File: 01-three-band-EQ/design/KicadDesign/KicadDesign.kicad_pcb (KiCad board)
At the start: 2 copper layers, 101 x 80.9 mm, 34 parts, among them J2 Output, J3 Input, J4 Supply, U1 TL072, U2 TL072, U3 TL072

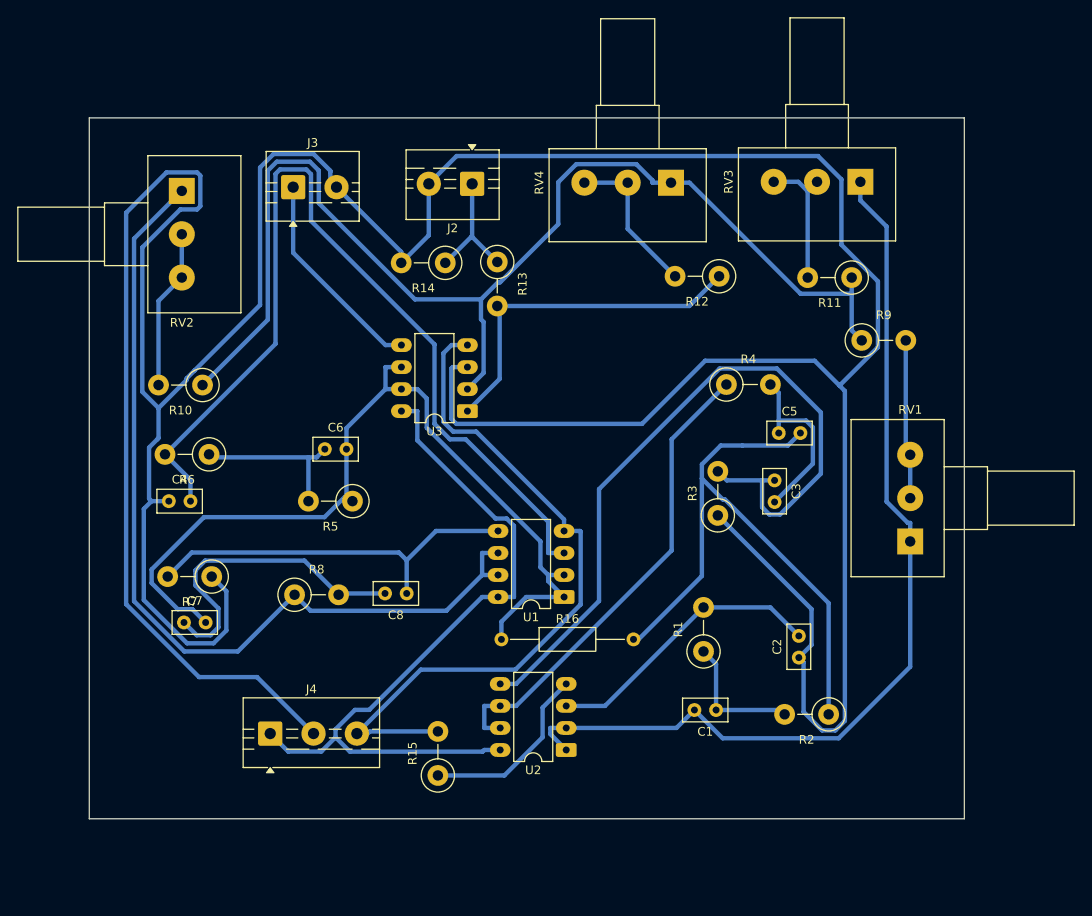
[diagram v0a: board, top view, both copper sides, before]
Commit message: feat: PCB routed
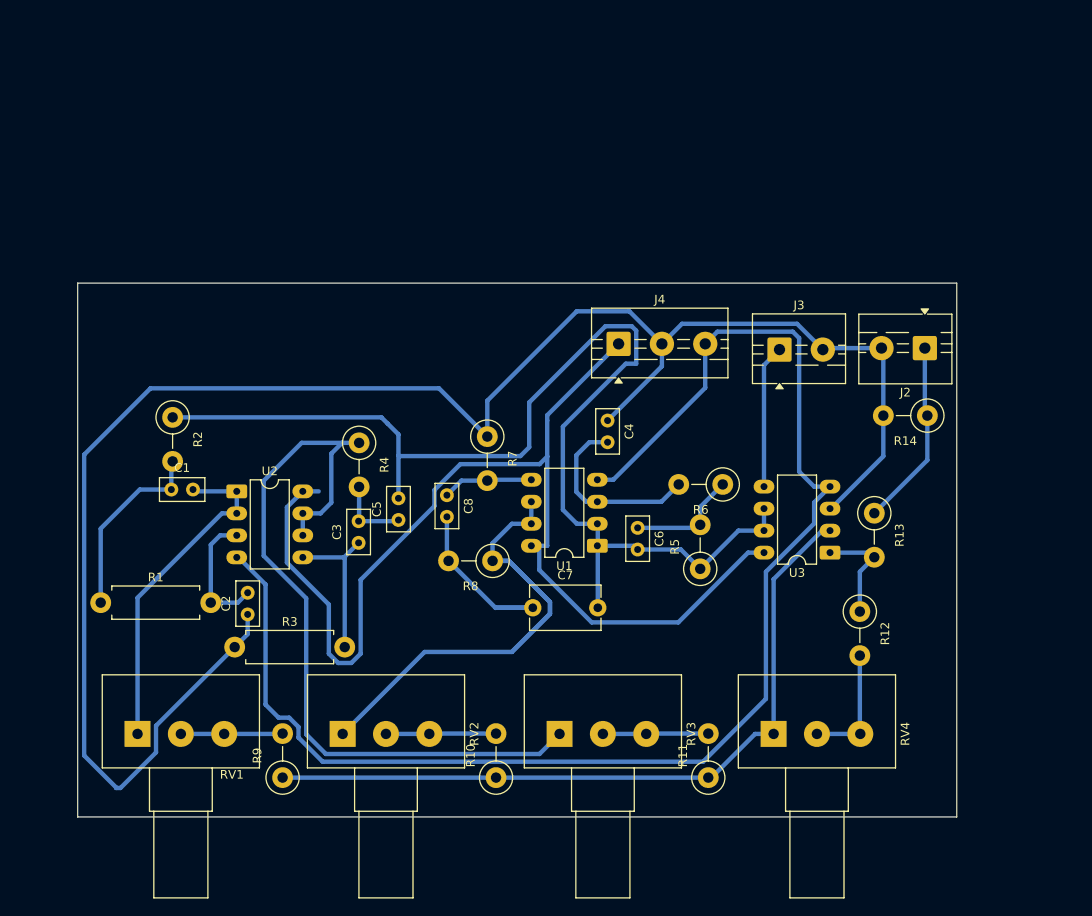
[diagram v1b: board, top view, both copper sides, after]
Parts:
- removed R15: 0, Resistor_THT:R_Axial_DIN0411_L9.9mm_D3.6mm_P5.08mm_Vertical
- removed R16: 270k, Resistor_THT:R_Axial_DIN0207_L6.3mm_D2.5mm_P15.24mm_Horizontal
- C7: footprint Capacitor_THT:C_Disc_D5.0mm_W2.5mm_P2.50mm -> Capacitor_THT:C_Disc_D8.0mm_W5.0mm_P7.50mm
- R1, R3: footprint Resistor_THT:R_Axial_DIN0411_L9.9mm_D3.6mm_P5.08mm_Vertical -> Resistor_THT:R_Axial_DIN0411_L9.9mm_D3.6mm_P12.70mm_Horizontal
- moved RV1 91.9 mm to (35.7, 98.5), turned to 90 degrees
- moved R9 83.7 mm to (52.4, 103.5), turned to 90 degrees
- moved R2 83.1 mm to (39.7, 61.9), turned to -90 degrees
- moved RV3 72.6 mm to (84.4, 98.5), turned to 90 degrees
- moved R1 69.8 mm to (31.4, 83.3), turned to 0 degrees
- moved C1 67.8 mm to (39.6, 70.3), turned to 0 degrees
- moved RV2 65.4 mm to (59.4, 98.5), turned to 90 degrees
- moved RV4 64.7 mm to (109.1, 98.5), turned to 90 degrees
- moved C2 63.8 mm to (48.4, 84.7)
- moved J4 60.3 mm to (91.2, 53.5)
- moved R11 60.0 mm to (101.5, 103.5), turned to 90 degrees
- moved R6 59.4 mm to (103.2, 69.7)
- moved J3 59.2 mm to (109.8, 54.1)
- moved R14 58.4 mm to (126.8, 61.7)
- moved R3 57.8 mm to (46.9, 88.4), turned to 0 degrees
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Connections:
- RV3 pad 1: /OUT_LP -> /OUT_HP
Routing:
- net GND: track 433.4 -> 209.0 mm
- net Net-(U1A-+): track 106.7 -> 21.6 mm
- net Net-(U2B-+): track 88.0 -> 17.5 mm
- net /OUT_LP: track 109.0 -> 38.9 mm
- net VEE: track 103.6 -> 163.5 mm
- net Net-(U3A--): track 139.1 -> 85.4 mm
- net VCC: track 85.3 -> 128.0 mm
- net /OUT_BP: track 103.6 -> 65.8 mm
- net /IN: track 172.2 -> 135.1 mm
- net Net-(U1B-+): track 44.9 -> 10.5 mm
- net /OUT_HP: track 55.2 -> 89.0 mm
- net Net-(R12-Pad1): track 40.8 -> 12.3 mm
- net Net-(U2A-+): track 32.9 -> 14.9 mm
- net Net-(C7-Pad1): track 36.7 -> 21.4 mm
- net Net-(C3-Pad2): track 20.7 -> 8.83 mm
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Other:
- board size 101 x 80.9 mm -> 101.4 x 61.6 mm

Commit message: feat: PCB routed
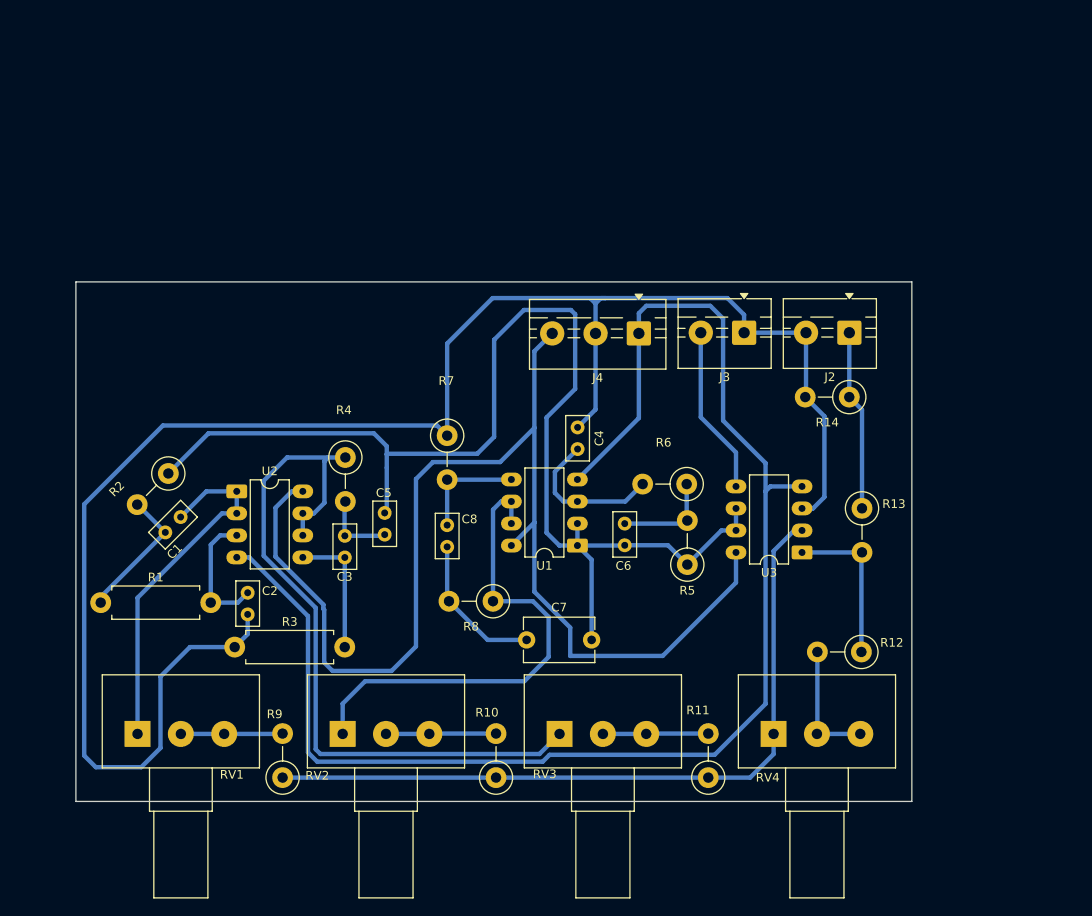
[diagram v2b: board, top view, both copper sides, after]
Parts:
- moved R14 9.26 mm to (117.8, 59.6)
- moved J2 8.89 mm to (117.8, 52.2)
- moved R2 6.50 mm to (39.2, 68.4), turned to -135 degrees
- moved C1 4.99 mm to (38.9, 75.2), turned to 45 degrees
- moved R12 4.66 mm to (119.2, 89.0), turned to 180 degrees
- moved R8 4.66 mm to (76.7, 83.2)
- moved R7 4.63 mm to (71.4, 64.0)
- moved J3 4.53 mm to (105.7, 52.2), turned to 180 degrees
- moved R6 4.16 mm to (99.1, 69.6)
- moved C7 3.78 mm to (80.6, 87.6)
- moved C4 3.55 mm to (86.5, 63.1)
- moved C8 3.46 mm to (71.4, 74.4)
- moved U3 3.23 mm to (112.4, 77.5)
- moved J4 2.63 mm to (93.5, 52.2), turned to 180 degrees
- moved C3 2.32 mm to (59.6, 78.1)
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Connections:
- J3 pad 1: /INPUT -> GND
- J3 pad 2: GND -> /INPUT
- J4 pad 1: VCC -> VEE
- J4 pad 3: VEE -> VCC
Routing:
- net VCC: track 128.0 -> 141.4 mm
- net /OUT_BP: track 65.8 -> 56.9 mm
- net Net-(R12-Pad1): track 12.3 -> 18.5 mm
- net Net-(C1-Pad1): track 21.9 -> 15.8 mm
- net /OUT_HP: track 89.0 -> 84.3 mm
- net /IN: track 135.1 -> 139.7 mm
- net Net-(U1A-+): track 21.6 -> 17.5 mm
- net Net-(C7-Pad1): track 21.4 -> 17.6 mm
- net GND: track 209.0 -> 205.5 mm
- net VEE: track 163.5 -> 166.5 mm
- net /INPUT: track 16.6 -> 19.4 mm
- net /OUT_LP: track 38.9 -> 41.4 mm
- net Net-(U2B-+): track 17.5 -> 15.2 mm
- net Net-(U1B-+): track 10.5 -> 12.7 mm
- net Net-(C6-Pad1): track 13.1 -> 11.6 mm
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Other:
- board size 101.4 x 61.6 mm -> 96.5 x 60 mm
